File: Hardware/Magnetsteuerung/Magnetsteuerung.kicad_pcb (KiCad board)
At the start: 2 copper layers, 90 x 98 mm, 200 parts, among them J1 Conn_02x08_Odd_Even, J10 OUT1, J11 OUT1, J12 OUT1, J13 OUT1, J14 OUT1, J15 OUT1, J16 OUT1, J17 OUT1, J18 OUT1, J19 OUT1, J2 OUT1, J20 OUT1, J21 OUT1, J3 OUT1, J4 OUT1, J5 OUT1, J6 OUT1, J7 OUT1, J8 OUT1, J9 OUT1, Q1 Q_NMOS_GSD, Q10 Q_NMOS_GSD, Q11 Q_NMOS_GSD, Q12 Q_NMOS_GSD, Q13 Q_NMOS_GSD, Q14 Q_NMOS_GSD, Q15 Q_NMOS_GSD, Q16 Q_NMOS_GSD, Q2 Q_NMOS_GSD, Q3 Q_NMOS_GSD, Q4 Q_NMOS_GSD, Q5 Q_NMOS_GSD, Q6 Q_NMOS_GSD, Q7 Q_NMOS_GSD, Q8 Q_NMOS_GSD, Q9 Q_NMOS_GSD, U1 TL2575, U10 IRS44273, U11 IRS44273, U12 IRS44273, U13 IRS44273, U14 IRS44273, U15 IRS44273, U16 IRS44273, U17 IRS44273, U2 IRS44273, U3 IRS44273, U4 IRS44273, U5 IRS44273, U6 IRS44273, U7 IRS44273, U8 IRS44273, U9 IRS44273

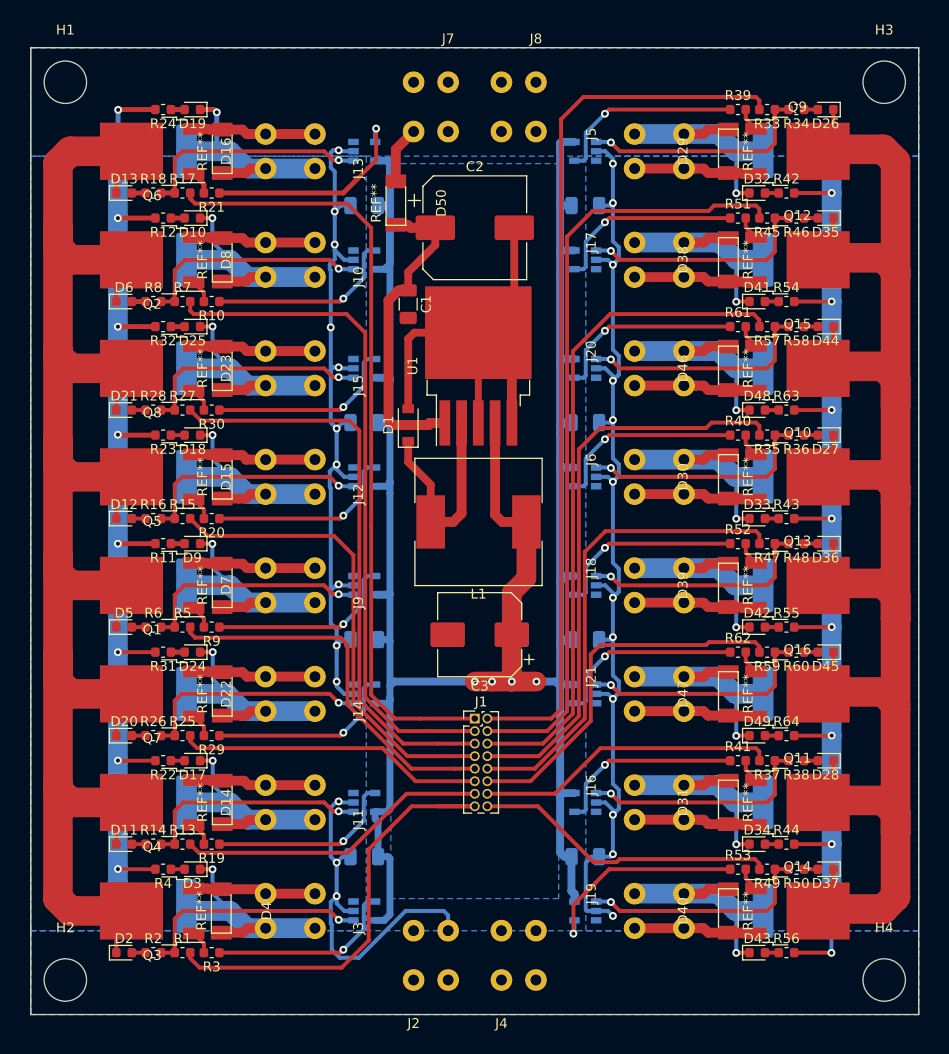
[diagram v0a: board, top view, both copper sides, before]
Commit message: update layout
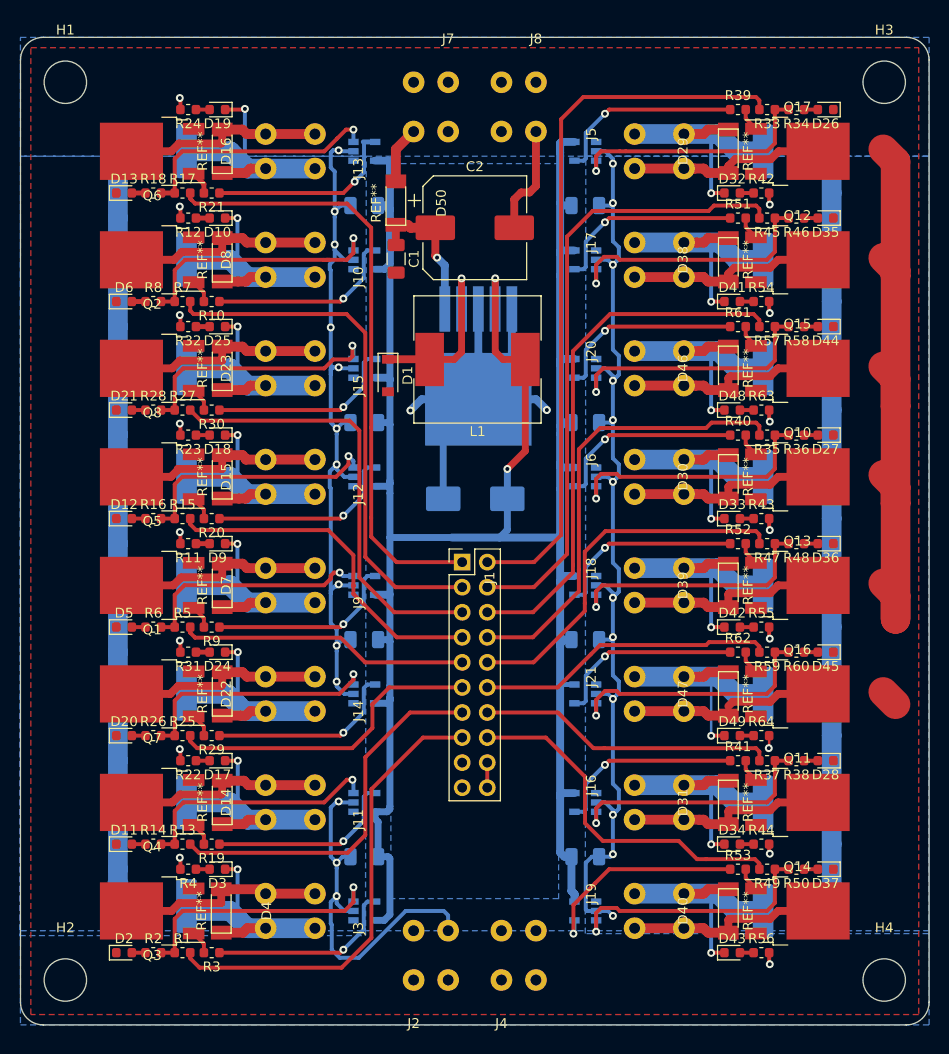
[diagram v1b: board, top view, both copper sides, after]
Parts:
- removed Q9: Q_NMOS_GSD, Package_TO_SOT_SMD:TO-252-2
- added Q17: Q_NMOS_GDS, Package_TO_SOT_SMD:TO-252-2, F.Cu at (167.7, 42.5)
- C3, U1: moved to B.Cu
- D3, D9: value LED -> LED_R
- J1: footprint Connector_PinHeader_1.27mm:PinHeader_2x08_P1.27mm_Vertical -> MK_Footprints:PinHeader_2x10_P2.54mm_61202022021
- R1, R13, R15, R17, R25, R27, R33, R35, R37, R45, R47, R49, R5, R57, R59, R7: value 10 -> 1.5k
- R14, R16, R18, R26, R28, R34, R36, R38, R46, R48, R50, R58, R6, R60, R8: value 2k -> 80
- R2: value 2k -> 1.5k
- U10, U11, U12, U13, U14, U15, U16, U17, U2, U3, U4, U5, U6, U7, U8, U9: value IRS44273 -> MCP1416R
- moved U5 33.0 mm to (123.8, 75.5)
- moved U6 33.0 mm to (123.8, 108.5)
- moved L1 16.5 mm to (135.3, 63.6)
- moved J1 15.9 mm to (133.7, 84.1), turned to 270 degrees
- moved C3 13.8 mm to (135.1, 77.7)
- moved D1 5.43 mm to (126.2, 65.2), turned to 270 degrees
- moved C1 4.76 mm to (127.0, 53.4)
- moved R11 2.54 mm to (106.0, 82.3)
- moved R12 2.54 mm to (106.0, 49.3)
- moved R22 2.54 mm to (106.0, 104.3)
- moved R23 2.54 mm to (106.0, 71.3)
- moved R24 2.54 mm to (106.0, 38.3)
- moved R31 2.54 mm to (106.0, 93.3)
- moved R32 2.54 mm to (106.0, 60.3)
- moved R4 2.54 mm to (106.0, 115.3)
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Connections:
- Q1 pad 2: GND -> Net-(D7-Pad2)
- Q1 pad 3: Net-(D7-Pad2) -> GND
- Q10 pad 2: GND -> Net-(D30-Pad2)
- Q10 pad 3: Net-(D30-Pad2) -> GND
- Q11 pad 2: GND -> Net-(D31-Pad2)
- Q11 pad 3: Net-(D31-Pad2) -> GND
- Q12 pad 2: GND -> Net-(D38-Pad2)
- Q12 pad 3: Net-(D38-Pad2) -> GND
- Q13 pad 2: GND -> Net-(D39-Pad2)
- Q13 pad 3: Net-(D39-Pad2) -> GND
- Q14 pad 2: GND -> Net-(D40-Pad2)
- Q14 pad 3: Net-(D40-Pad2) -> GND
- Q15 pad 2: GND -> Net-(D46-Pad2)
- Q15 pad 3: Net-(D46-Pad2) -> GND
- Q16 pad 2: GND -> Net-(D47-Pad2)
- Q16 pad 3: Net-(D47-Pad2) -> GND
- Q2 pad 2: GND -> Net-(D8-Pad2)
- Q2 pad 3: Net-(D8-Pad2) -> GND
- Q3 pad 2: GND -> Net-(D4-Pad2)
- Q3 pad 3: Net-(D4-Pad2) -> GND
- Q4 pad 2: GND -> Net-(D14-Pad2)
- Q4 pad 3: Net-(D14-Pad2) -> GND
- Q5 pad 2: GND -> Net-(D15-Pad2)
- Q5 pad 3: Net-(D15-Pad2) -> GND
- Q6 pad 2: GND -> Net-(D16-Pad2)
- Q6 pad 3: Net-(D16-Pad2) -> GND
- Q7 pad 2: GND -> Net-(D22-Pad2)
- Q7 pad 3: Net-(D22-Pad2) -> GND
- Q8 pad 2: GND -> Net-(D23-Pad2)
- Q8 pad 3: Net-(D23-Pad2) -> GND
- U10 pad 1: Net-(R33-Pad1) -> (no net)
- U10 pad 3: (no net) -> Net-(R33-Pad1)
- U11 pad 1: Net-(R35-Pad1) -> (no net)
- U11 pad 3: (no net) -> Net-(R35-Pad1)
- U12 pad 1: Net-(R37-Pad1) -> (no net)
- U12 pad 3: (no net) -> Net-(R37-Pad1)
- U13 pad 1: Net-(R45-Pad1) -> (no net)
- U13 pad 3: (no net) -> Net-(R45-Pad1)
- U14 pad 1: Net-(R47-Pad1) -> (no net)
- U14 pad 3: (no net) -> Net-(R47-Pad1)
- U15 pad 1: Net-(R49-Pad1) -> (no net)
- U15 pad 3: (no net) -> Net-(R49-Pad1)
- U16 pad 1: Net-(R57-Pad1) -> (no net)
- U16 pad 3: (no net) -> Net-(R57-Pad1)
- U17 pad 1: Net-(R59-Pad1) -> (no net)
- U17 pad 3: (no net) -> Net-(R59-Pad1)
- U2 pad 1: Net-(R5-Pad1) -> (no net)
- U2 pad 3: (no net) -> Net-(R5-Pad1)
- U3 pad 1: Net-(R7-Pad1) -> (no net)
- U3 pad 3: (no net) -> Net-(R7-Pad1)
- U4 pad 1: Net-(R1-Pad1) -> (no net)
- U4 pad 3: (no net) -> Net-(R1-Pad1)
- U5 pad 1: Net-(R13-Pad1) -> (no net)
- U5 pad 3: (no net) -> Net-(R15-Pad1)
- U5 pad 4: Net-(R19-Pad1) -> Net-(R20-Pad1)
- U6 pad 1: Net-(R15-Pad1) -> (no net)
- U6 pad 3: (no net) -> Net-(R13-Pad1)
- U6 pad 4: Net-(R20-Pad1) -> Net-(R19-Pad1)
- U7 pad 1: Net-(R17-Pad1) -> (no net)
- U7 pad 3: (no net) -> Net-(R17-Pad1)
- U8 pad 1: Net-(R25-Pad1) -> (no net)
- U8 pad 3: (no net) -> Net-(R25-Pad1)
- U9 pad 1: Net-(R27-Pad1) -> (no net)
- U9 pad 3: (no net) -> Net-(R27-Pad1)
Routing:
- net GND: track 638.8 -> 342.2 mm, vias 25 -> 27
- net +48V: track 228.6 -> 178.3 mm
- net Net-(C1-Pad1): track 37.8 -> 14.8 mm, vias 0 -> 1
- net IN8: track 79.2 -> 61.8 mm
- net IN9: track 89.7 -> 72.9 mm
- net IN7: track 69.6 -> 53.9 mm
- net IN10: track 78.9 -> 63.5 mm
- net IN6: track 58.8 -> 44.8 mm
- net IN11: track 68.1 -> 54.2 mm
- net IN12: track 58.5 -> 46.1 mm
- net IN5: track 47.7 -> 35.3 mm
- net IN13: track 48.5 -> 37.7 mm
- net IN4: track 38.7 -> 29.4 mm
- net Net-(D15-Pad2): track 12.6 -> 21.4 mm
- net Net-(D23-Pad2): track 12.5 -> 20.5 mm
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- added copper zone on B.Cu, net GND
- removed copper zone on B.Cu, net +12V
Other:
- board size 90 x 98 mm -> 92.1 x 100.1 mm
